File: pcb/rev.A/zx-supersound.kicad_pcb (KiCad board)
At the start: 2 copper layers, 170 x 63.6 mm, 166 parts, among them J1 PJ307, J2 PinHeader, J3 Conn_01x04, J4 Conn_02x31_Row_Letter_First, J5 Conn_01x04, SW2 SW_DIP_x05, U1 MCP602, U10 YM3014B, U11 SAM2695, U12 AS6C4008-55SIN, U13 AMS1117-3.3, U14 SAA1099, U16 AMS1117-3.3, U17 NCP1117-5.0_TO252, U2 MCP602, U20 NCP1117-5.0_TO252, U21 NCP1117-5.0_TO252, U22 AS6C4008-55SIN, U23 74HC245, U3 Z84C0020PEC, U4 YM2203, U5 YM3014B, U6 MCP602, U7 EPM3256ATC144, U8 27C512, U9 YM2203, X1 32MHz

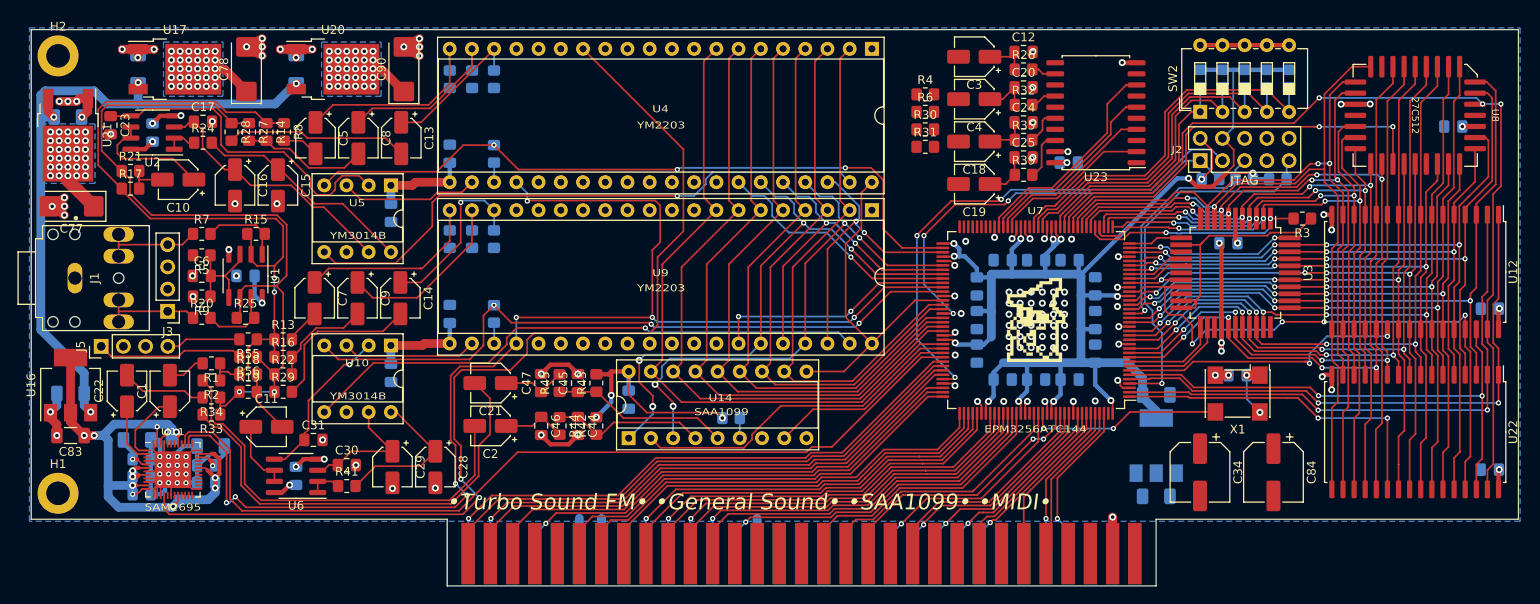
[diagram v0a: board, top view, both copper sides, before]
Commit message: wip pcb rev.A
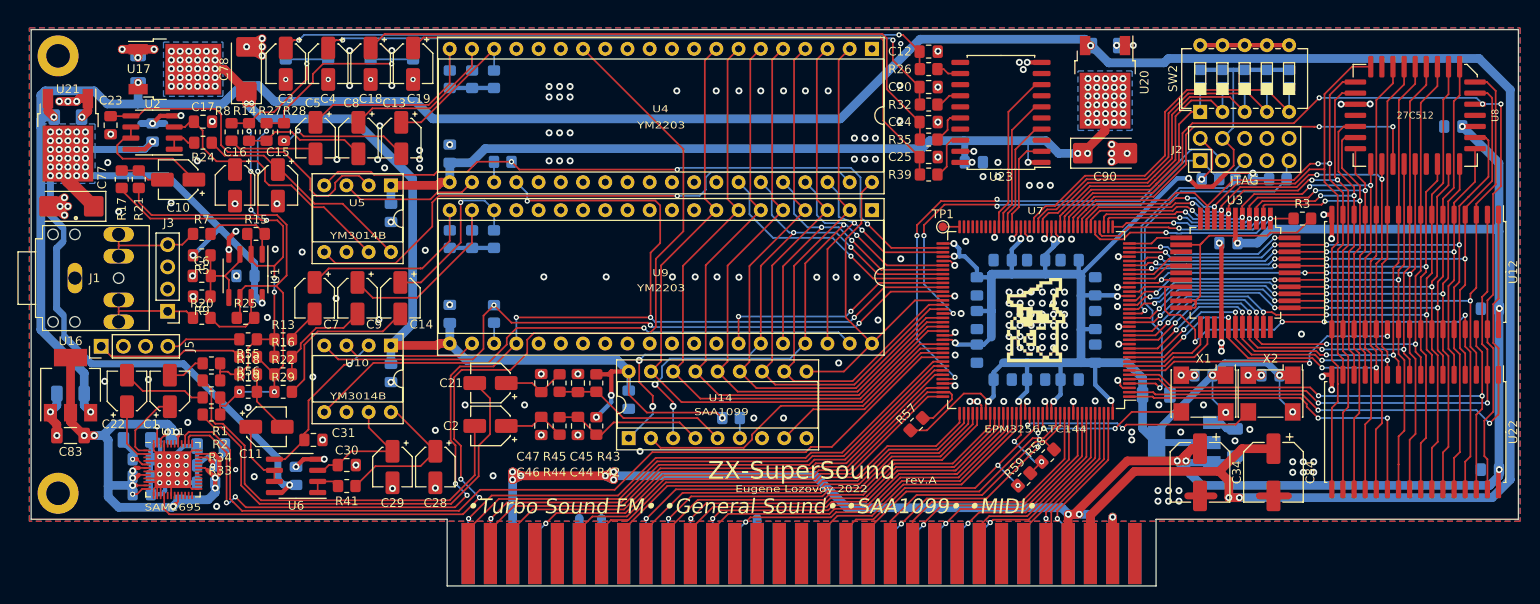
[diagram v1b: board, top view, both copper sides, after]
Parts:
- added C37: 100n, Capacitor_SMD:C_0805_2012Metric_Pad1.18x1.45mm_HandSolder, B.Cu at (200.3, 101.1)
- added R57: 10k, Resistor_SMD:R_0805_2012Metric_Pad1.20x1.40mm_HandSolder, F.Cu at (159.8, 106.7)
- added R58: 10k, Resistor_SMD:R_0805_2012Metric_Pad1.20x1.40mm_HandSolder, F.Cu at (174.8, 110.3)
- added R59: 24k, Resistor_SMD:R_0805_2012Metric_Pad1.20x1.40mm_HandSolder, F.Cu at (172.1, 113.0)
- added TP1: TestPoint, TestPoint:TestPoint_Pad_D1.0mm, F.Cu at (162.8, 84.1)
- added X2: ??MHz, Oscillator:Oscillator_SMD_SeikoEpson_SG8002CA-4Pin_7.0x5.0mm, F.Cu at (200.3, 103.2)
- R30, R31, R4, R6: moved to B.Cu
- moved C98 92.5 mm to (181.3, 63.4), turned to 0 degrees
- moved U20 88.3 mm to (181.3, 67.6), turned to -90 degrees
- moved C90 80.7 mm to (181.3, 75.7), turned to 0 degrees
- moved C3 78.7 mm to (87.7, 65.5), turned to -90 degrees
- moved C4 74.0 mm to (92.5, 65.5), turned to -90 degrees
- moved R4 73.2 mm to (87.7, 66.0), turned to -90 degrees
- moved C18 69.6 mm to (97.4, 65.5), turned to -90 degrees
- moved R6 68.4 mm to (92.5, 66.0), turned to -90 degrees
- moved C19 65.6 mm to (102.2, 65.5), turned to -90 degrees
- moved R30 63.8 mm to (97.4, 66.0), turned to -90 degrees
- moved R31 59.2 mm to (102.2, 66.0), turned to -90 degrees
- moved C35 10.9 mm to (196.2, 108.8), turned to 90 degrees
- moved U23 10.9 mm to (169.4, 71.1)
- moved C12 10.9 mm to (161.2, 64.1)
- moved C20 10.9 mm to (161.2, 68.2)
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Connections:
- net ~{IORQGE1} renamed ~{IORQGE}
- C88 pad 2: +5V -> +3V3
- H1 pad 1: unconnected-(H1-Pad1) -> GND
- H2 pad 1: unconnected-(H2-Pad1) -> GND
- J4 pad b20: unconnected-(J4-Padb20) -> ~{IODOS}
- U7 pad 125: unconnected-(U7-Pad125) -> /CLKx
- U7 pad 132: ~{WAIT} -> ~{IODOS}
- U7 pad 133: A7 -> ~{WAIT}
- U7 pad 134: A6 -> A7
- U7 pad 136: A5 -> A6
- U7 pad 137: ~{M1} -> A5
- U7 pad 138: A4 -> ~{M1}
- U7 pad 139: A8 -> A4
- U7 pad 140: A9 -> A8
- U7 pad 141: A10 -> A9
- U7 pad 142: A11 -> A10
- U7 pad 143: unconnected-(U7-Pad143) -> A11
- U7 pad 2: /GMA16 -> /GMA17
- U7 pad 5: /GMA17 -> /GMA16
- U7 pad 72: unconnected-(U7-Pad72) -> Net-(TP1-Pad1)
- X1 pad 1: +5V -> +3V3
- X1 pad 4: +5V -> +3V3
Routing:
- net +12V: track 78.3 -> 335.8 mm, vias 4 -> 6
- net +5V: track 43.0 -> 271.9 mm, vias 6 -> 14
- net +5VA: track 15.6 -> 107.3 mm, vias 33 -> 34
- net +5VA_1: track 19.6 -> 100.5 mm, vias 31 -> 34
- net /GCH0: track 5.04 -> 75.9 mm, vias 0 -> 2
- net +5VA_2: track 44.8 -> 113.3 mm, vias 33 -> 35
- net /GCH1: track 5.37 -> 73.7 mm, vias 0 -> 2
- net /GCH2: track 4.94 -> 73.0 mm
- net /GCH3: track 5.29 -> 71.5 mm
- net +3V3: track 168.1 -> 229.6 mm, vias 13 -> 19
- net ~{IODOS}: track 0.00 -> 30.5 mm
- net /CLKx: track 0.00 -> 27.8 mm, vias 0 -> 2
- net GND: track 217.8 -> 231.4 mm, vias 139 -> 250
- net /GDAC3: track 18.3 -> 11.0 mm
- net /GDAC2: track 19.9 -> 13.2 mm
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- added copper zone on F.Cu, net GND
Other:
- board text added: "Eugene Lozovoy 2022"
- board text added: "ZX-SuperSound"
- board text added: "rev.A"
